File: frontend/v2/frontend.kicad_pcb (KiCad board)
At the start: 2 copper layers, 41.5 x 49.9 mm, 122 parts, among them CN1 EDGE, CN2 BREAKOUT, CN3 TXL, CN4 AGND, CN5 AGND, J1 0, J2 0, P1 BNC, P2 BNC, T1 4:1, T2 8:1

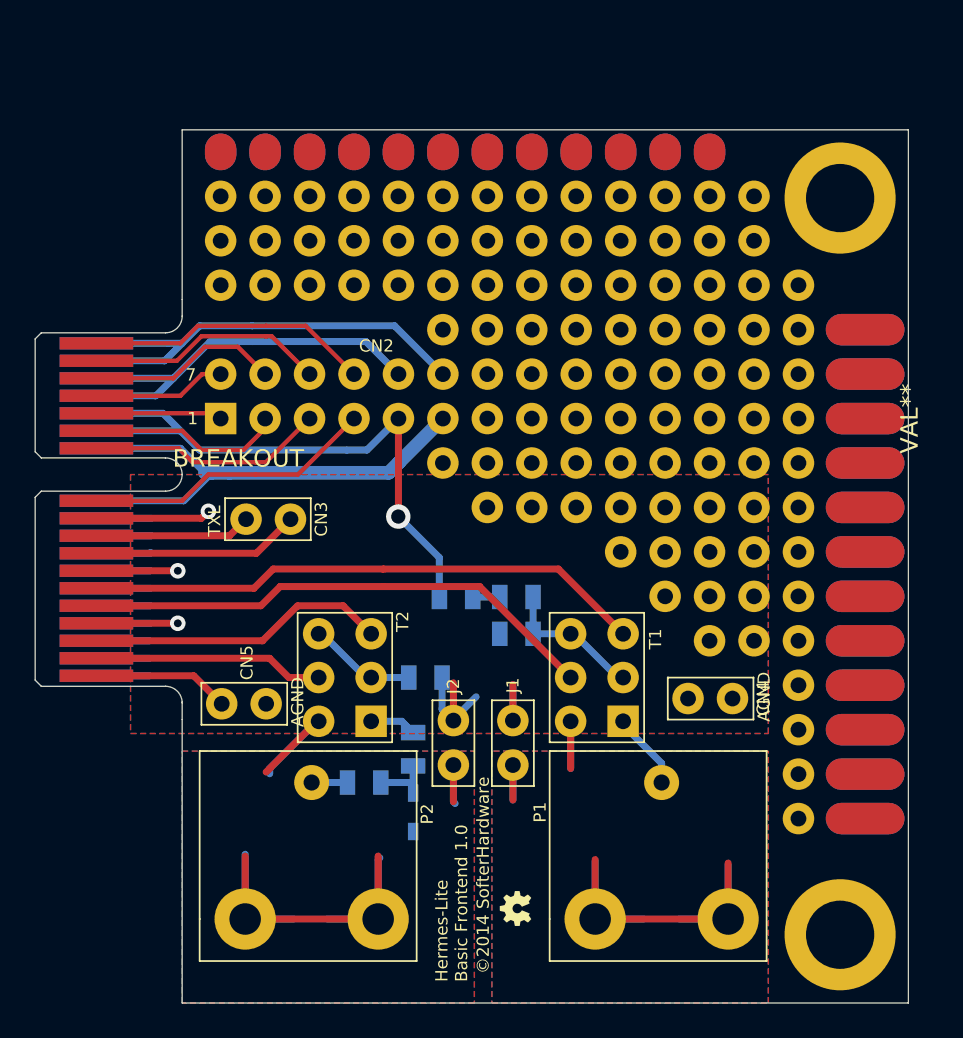
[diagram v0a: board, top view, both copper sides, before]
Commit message: Updated Schematic, floorplanning
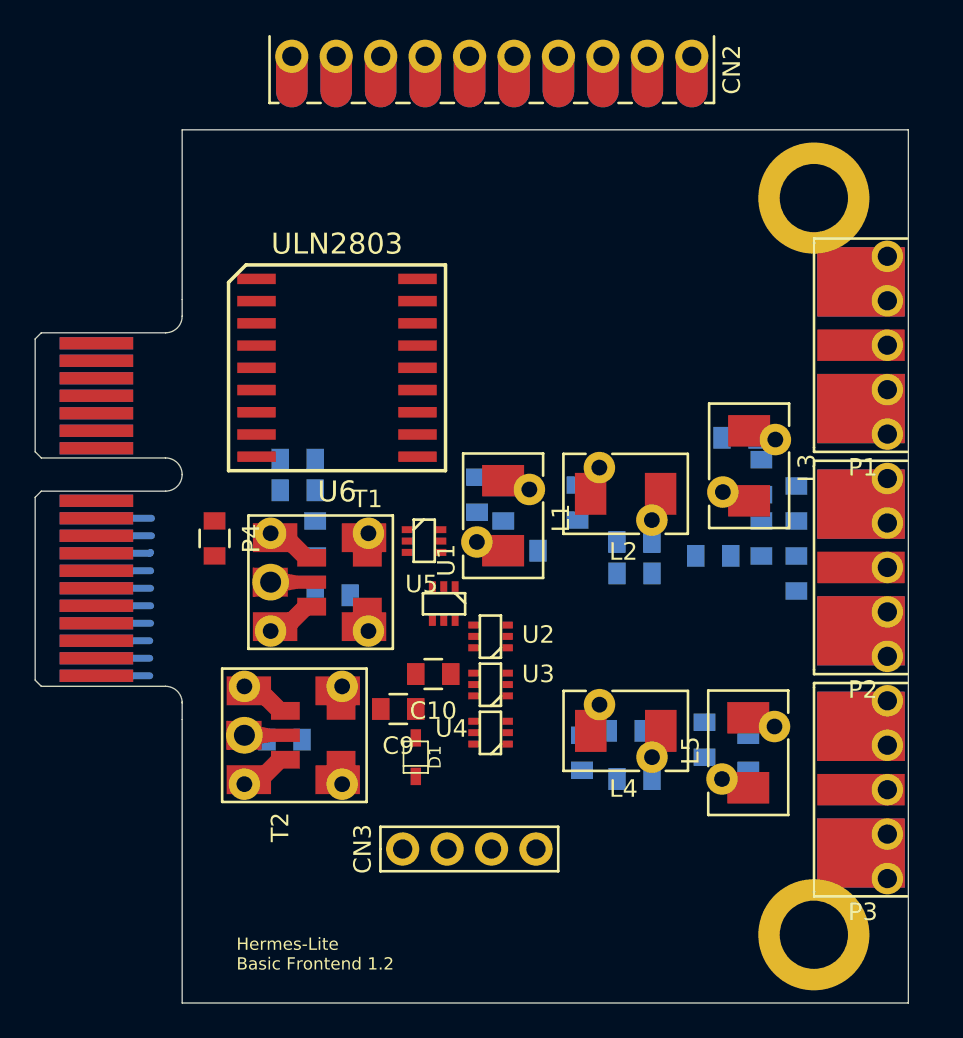
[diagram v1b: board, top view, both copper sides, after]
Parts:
- removed CN4, CN5: AGND, HERMESLITE:JUMPER
- removed G*** (x2): OSHW-logo_silkscreen-front_2mm, OSHW:OSHW-logo_silkscreen-front_2mm
- removed HOLE (x98): VAL**, HERMESLITE:HOLE
- removed J1, J2: 0, HERMESLITE:JUMPER
- removed PROTOEDGE12L: VAL**, HERMESLITE:PROTOEDGE12L
- removed PROTOEDGE12S: VAL**, HERMESLITE:PROTOEDGE12S
- added C10: 0.1uF, Capacitors_SMD:C_0805, F.Cu at (113.8, 103.5)
- added C11: 0pF, Capacitors_SMD:C_0805, B.Cu at (122.2, 108.0)
- added C12: 0pF, Capacitors_SMD:C_0805, B.Cu at (125.2, 109.5)
- added C13: 0pF, Capacitors_SMD:C_0805, B.Cu at (129.2, 107.2)
- added C14: 0pF, Capacitors_SMD:C_0805, B.Cu at (124.8, 106.8)
- added C15: 0pF, Capacitors_SMD:C_0805, B.Cu at (131.8, 108.0)
- added C5: 8.4pF, Capacitors_SMD:C_0805, B.Cu at (116.2, 93.2)
- added C6: 75pF, Capacitors_SMD:C_0805, B.Cu at (117.8, 93.8)
- added C7: 0.1uF, Capacitors_SMD:C_0805, B.Cu at (108.0, 99.0)
- added C8: 0.1uF, Capacitors_SMD:C_0805, B.Cu at (105.2, 107.2)
- added C9: 0.1uF, Capacitors_SMD:C_0805, F.Cu at (111.8, 105.5)
- added L1: 150nH, HERMESLITE:inductor, F.Cu at (117.7, 94.5)
- added L2: 270nH, HERMESLITE:inductor, F.Cu at (124.7, 93.2)
- added L3: 0H, HERMESLITE:inductor, F.Cu at (131.8, 91.6)
- added L4: 0nH, HERMESLITE:inductor, F.Cu at (124.8, 106.8)
- added L5: 0nH, HERMESLITE:inductor, F.Cu at (131.8, 108.0)
- added P3: SMA/BNC/HDR, HERMESLITE:rfconnector, F.Cu at (140.8, 110.1)
- added P4: CONN_01X02, Capacitors_SMD:C_0805, F.Cu at (101.2, 95.8)
- added R2: DNI, Capacitors_SMD:C_0805, B.Cu at (106.0, 93.0)
- added R3: DNI, Capacitors_SMD:C_0805, B.Cu at (125.2, 97.8)
- added R4: 0, Capacitors_SMD:C_0805, B.Cu at (129.8, 96.8)
- added R5: 87, Capacitors_SMD:C_0805, B.Cu at (134.5, 97.8)
- added R6: 43, Capacitors_SMD:C_0805, B.Cu at (132.5, 95.8)
- added R7: 2.2K, Capacitors_SMD:C_0805, B.Cu at (132.5, 92.2)
- added R8: 76, Capacitors_SMD:C_0805, B.Cu at (134.5, 93.8)
- added U1: PE4259, HERMESLITE:pe4259, F.Cu at (115.0, 98.5)
- added U2: PE4259, HERMESLITE:pe4259, F.Cu at (118.0, 102.0)
- added U3: PE4259, HERMESLITE:pe4259, F.Cu at (118.0, 104.8)
- added U4: PE4259, HERMESLITE:pe4259, F.Cu at (118.0, 107.5)
- added U5: PE4259, HERMESLITE:pe4259, F.Cu at (112.2, 95.2)
- added U6: ULN2803, HERMESLITE:PSOP-18, F.Cu at (108.2, 86.0)
- C1: value 0.1 uF -> 110pF; footprint SMD_Packages:SMD-0805 -> Capacitors_SMD:C_0805
- C2: value 0.1 uF -> 220pF; footprint SMD_Packages:SMD-0805 -> Capacitors_SMD:C_0805
- C3: value 0.1 uF -> 160pF; footprint SMD_Packages:SMD-0805 -> Capacitors_SMD:C_0805
- C4: value 0.1 uF -> DNI; footprint SMD_Packages:SMD-0805 -> Capacitors_SMD:C_0805
- CN2: value BREAKOUT -> RELAYCNT; footprint HERMESLITE:BREAKOUT -> HERMESLITE:10pin
- CN3: value TXL -> RXCNT; footprint HERMESLITE:JUMPER -> HERMESLITE:4pinmid
- D1: moved to F.Cu
- FB1, R1: footprint SMD_Packages:SMD-0805 -> Capacitors_SMD:C_0805
- P1, P2: value BNC -> SMA/BNC/HDR; footprint HERMESLITE:BNCRA -> HERMESLITE:rfconnector
- T1: value 4:1 -> 1:1; footprint HERMESLITE:TRANSFREV -> HERMESLITE:TRANSFSMT
- T2: value 8:1 -> 8:1 Z; footprint HERMESLITE:TRANSFREV -> HERMESLITE:TRANSFSMT
- moved P2 39.5 mm to (140.8, 97.4)
- moved P1 35.7 mm to (140.8, 84.7)
- moved CN2 34.7 mm to (128.5, 67.1), turned to 90 degrees
- moved C4 29.1 mm to (131.2, 90.0), turned to 180 degrees
- moved CN3 20.9 mm to (112.0, 113.5)
- moved C3 17.3 mm to (125.2, 96.0), turned to 180 degrees
- moved T1 16.4 mm to (107.2, 98.2), turned to 90 degrees
- moved R1 14.8 mm to (106.0, 91.2), turned to 0 degrees
- moved C2 13.2 mm to (122.0, 93.7), turned to 270 degrees
- moved FB1 8.72 mm to (107.0, 95.8), turned to 90 degrees
- moved C1 4.75 mm to (118.7, 96.5), turned to 0 degrees
- moved D1 3.15 mm to (112.8, 108.2)
- moved T2 1.66 mm to (105.8, 107.0), turned to 90 degrees
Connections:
- C3 pad 2: Net-(C3-Pad2) -> GND
- C4 pad 2: Net-(C3-Pad1) -> GND
- CN1 pad A12: Net-(CN1-PadA11) -> Net-(CN1-PadA12)
- CN1 pad A13: Net-(CN1-PadA13) -> 5V
- CN1 pad A14: Net-(CN1-PadA13) -> 5V
- CN1 pad A15: Net-(CN1-PadA15) -> 3V
- CN1 pad A16: Net-(CN1-PadA15) -> 3V
- CN1 pad A17: Net-(CN1-PadA17) -> GNDREF
- CN1 pad A18: Net-(CN1-PadA17) -> GNDREF
- CN2 pad 1: Net-(CN1-PadB14) -> Net-(CN2-Pad1)
- CN2 pad 10: Net-(CN1-PadB18) -> GNDREF
- CN2 pad 2: Net-(CN1-PadB13) -> Net-(CN2-Pad2)
- CN2 pad 3: Net-(CN1-PadB12) -> Net-(CN2-Pad3)
- CN2 pad 4: Net-(CN1-PadB11) -> Net-(CN2-Pad4)
- CN2 pad 5: Net-(CN1-PadA13) -> Net-(CN2-Pad5)
- CN2 pad 6: Net-(CN1-PadA11) -> Net-(CN2-Pad6)
- CN2 pad 7: Net-(CN1-PadB15) -> Net-(CN2-Pad7)
- CN2 pad 8: Net-(CN1-PadB16) -> Net-(CN2-Pad8)
- CN2 pad 9: Net-(CN1-PadB17) -> Net-(CN2-Pad9)
- CN3 pad 1: Net-(CN1-PadB9) -> TR
- CN3 pad 2: Net-(CN1-PadB8) -> TAP
- D1 pad 1: Net-(C3-Pad1) -> Net-(C10-Pad2)
- D1 pad 2: Net-(D1-Pad2) -> GND
- FB1 pad 1: Net-(CN1-PadA13) -> Net-(C7-Pad1)
- P1 pad 1: Net-(P1-Pad1) -> Net-(C4-Pad1)
- P1 pad 2: Net-(J1-Pad1) -> GND
- P2 pad 1: Net-(C4-Pad1) -> Net-(P2-Pad1)
- P2 pad 2: Net-(D1-Pad2) -> GND
- R1 pad 1: Net-(C1-Pad1) -> 3V
- T1 pad 1: Net-(P1-Pad1) -> Net-(CN1-PadB6)
- T1 pad 2: Net-(J1-Pad1) -> Net-(C7-Pad1)
- T1 pad 3: Net-(C1-Pad1) -> Net-(CN1-PadB5)
- T1 pad 4: Net-(CN1-PadB5) -> GND
- T1 pad 5: Net-(CN1-PadB6) -> Net-(T1-Pad5)
- T2 pad 1: Net-(C3-Pad2) -> Net-(CN1-PadB3)
- T2 pad 2: Net-(D1-Pad2) -> Net-(C8-Pad1)
- T2 pad 3: Net-(C2-Pad1) -> Net-(CN1-PadB2)
- T2 pad 4: Net-(CN1-PadB2) -> GND
- T2 pad 5: Net-(CN1-PadB3) -> Net-(C9-Pad2)
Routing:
- net Net-(D1-Pad2): track 40.4 -> 0.00 mm
- net Net-(J1-Pad1): track 35.6 -> 0.00 mm
- net Net-(CN1-PadA13): track 34.9 -> 0.00 mm, vias 1 -> 0
- net GND: track 65.5 -> 31.0 mm, vias 3 -> 0
- net Net-(CN1-PadB6): track 32.1 -> 0.00 mm
- net Net-(CN1-PadB5): track 29.7 -> 0.00 mm
- net Net-(CN1-PadA11): track 28.9 -> 0.00 mm
- net Net-(CN1-PadA17): track 26.7 -> 0.00 mm
- net Net-(CN1-PadA15): track 23.7 -> 0.00 mm
- net Net-(CN1-PadB3): track 17.2 -> 0.00 mm
- net Net-(CN1-PadB11): track 16.7 -> 0.00 mm
- net Net-(CN1-PadB18): track 16.3 -> 0.00 mm
- net Net-(CN1-PadB17): track 13.7 -> 0.00 mm
- net Net-(CN1-PadB12): track 13.5 -> 0.00 mm
- net Net-(CN1-PadB2): track 13.5 -> 0.00 mm
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- removed copper zone on B.Cu, net GND
- removed copper zone on F.Cu, net GND
- removed copper zone on B.Cu, net Net-(D1-Pad2)
- removed copper zone on F.Cu, net Net-(D1-Pad2)
- removed copper zone on B.Cu, net Net-(J1-Pad1)
- removed copper zone on F.Cu, net Net-(J1-Pad1)
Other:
- board text added: "Hermes-Lite Basic Frontend 1.2"
- board text removed: "Hermes-Lite Basic Frontend 1.0"
- board text removed: "©2014 SofterHardware"
